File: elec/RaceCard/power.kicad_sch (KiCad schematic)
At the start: 26 parts, among them J2 UJC-H-G-SMT-2-P6-TR, J3 530480210, Q1 DMP3125L-7, U3 MCP73812T-420I_OT, U4 TLV74033PDQNR, U5 AS11AH

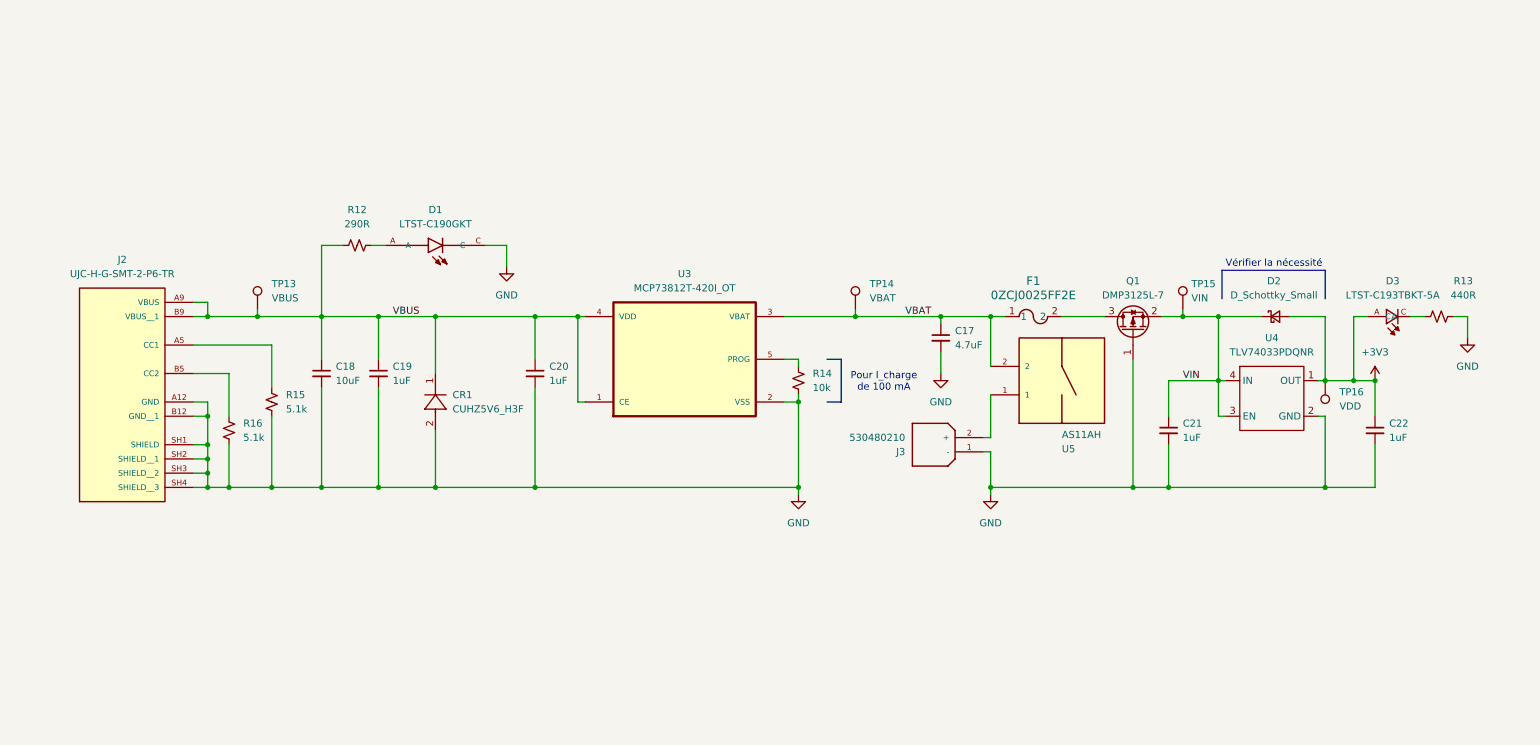
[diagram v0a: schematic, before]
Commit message: Cleanup
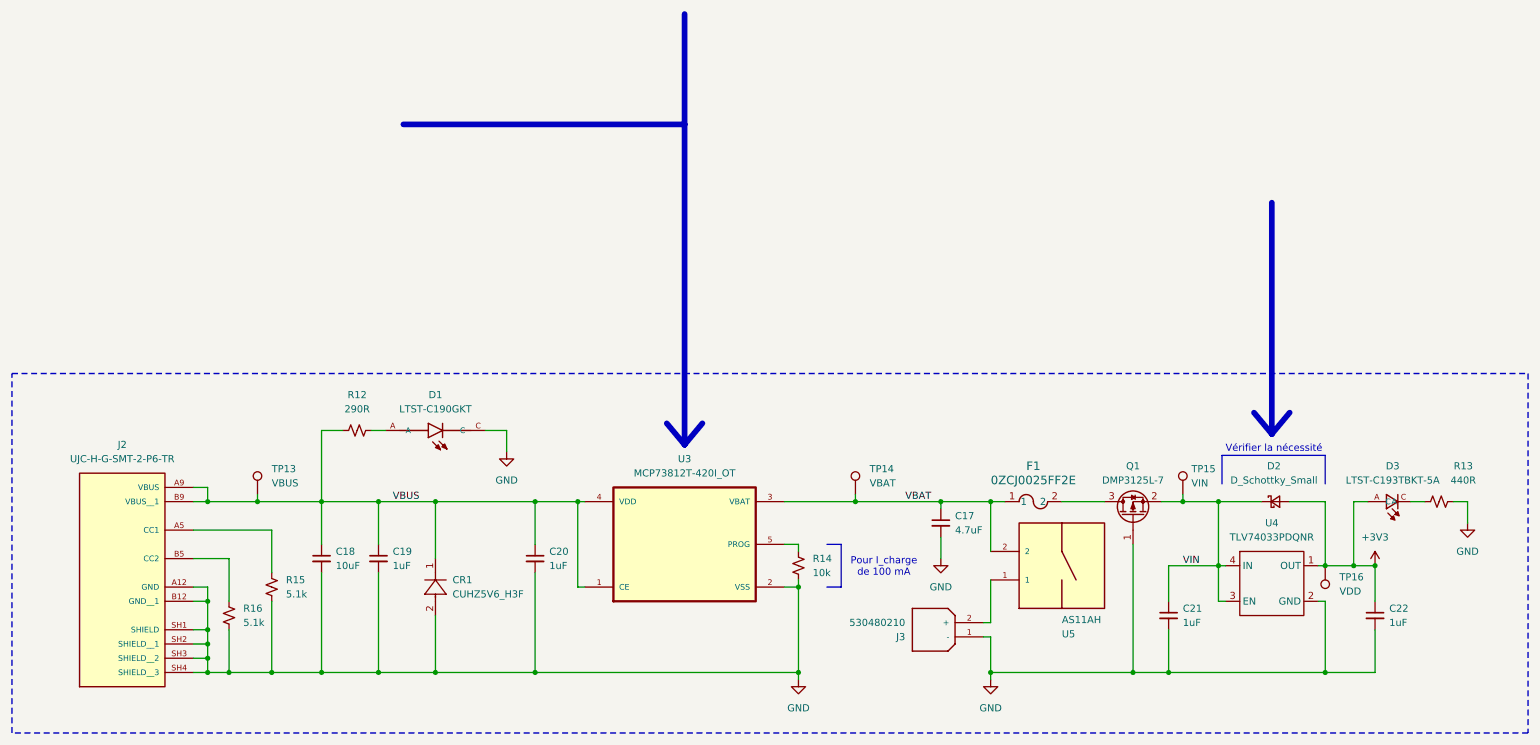
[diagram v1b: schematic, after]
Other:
- moved on the sheet: C17, C18, C19, C20, C21, C22, CR1, D1, D2, D3, F1, J2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
